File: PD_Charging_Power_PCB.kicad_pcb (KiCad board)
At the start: 2 copper layers, 30 x 28 mm, 35 parts, among them J1 105450-0101, Q1 CJQ4459, Q2 2N7002KDW, U1 STUSB4500

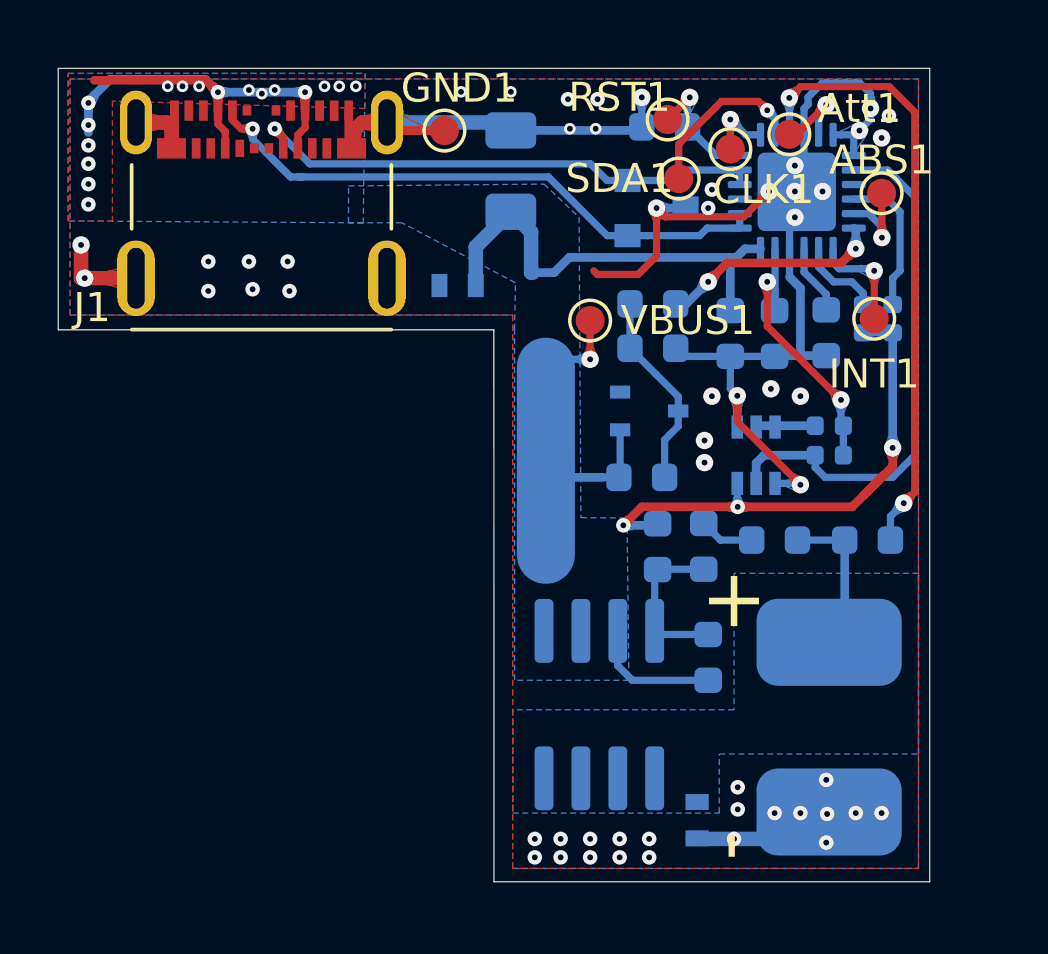
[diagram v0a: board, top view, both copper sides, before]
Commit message: Ruan: V0.3
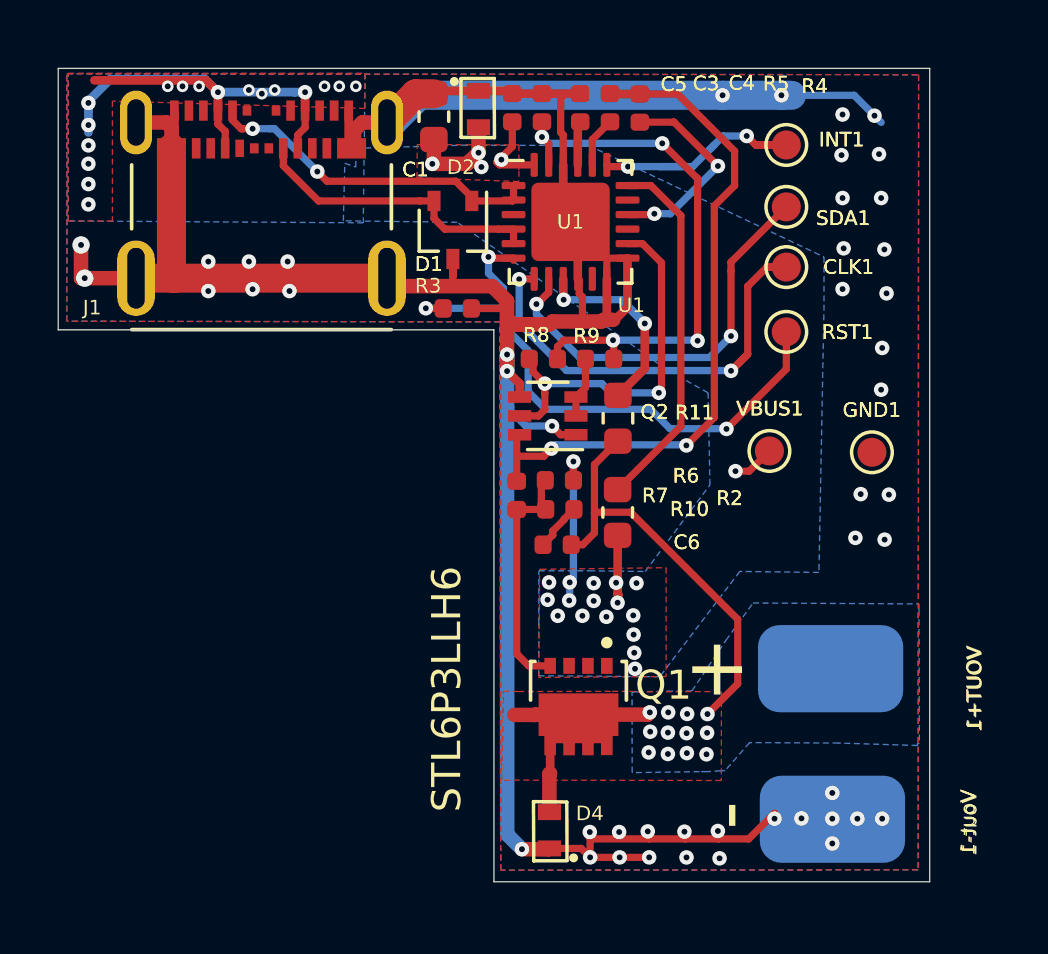
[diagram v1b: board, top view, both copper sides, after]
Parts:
- removed ABS1: ABS, TestPoint:TestPoint_Pad_D1.0mm
- removed Att1: ATT, TestPoint:TestPoint_Pad_D1.0mm
- removed C2: 1uF, Capacitor_SMD:C_0603_1608Metric
- removed D3: BAT54W, Package_TO_SOT_SMD:SOT-323_SC-70
- removed R1: 470R, Resistor_SMD:R_0603_1608Metric
- C1: footprint Capacitor_SMD:C_1206_3216Metric -> Capacitor_SMD:C_0603_1608Metric; moved to F.Cu
- C3, C4, C5, C6: footprint Capacitor_SMD:C_0603_1608Metric -> Capacitor_SMD:C_0402_1005Metric; moved to F.Cu
- D1: value ESD24VC2 -> ESDA25W; footprint Package_TO_SOT_SMD:SOT-23 -> Package_TO_SOT_SMD:SOT-323_SC-70; moved to F.Cu
- D2, D4, Q2, R11, R2, R4, R5, R8, R9, U1: moved to F.Cu
- Q1: value CJQ4459 -> STL6P3LLH6; footprint RuanProject:SOP-8_CJQ4459 -> RuanProject:PowerFLAT-3x3mm-8pin; moved to F.Cu
- R10, R3, R6, R7: footprint Resistor_SMD:R_0603_1608Metric -> Resistor_SMD:R_0402_1005Metric; moved to F.Cu
- moved GND1 18.4 mm to (63.2, 150.3)
- moved C4 11.5 mm to (53.1, 138.4), turned to 270 degrees
- moved R5 11.3 mm to (54.2, 138.4), turned to 270 degrees
- moved R4 11.3 mm to (55.2, 138.4), turned to 270 degrees
- moved C3 11.2 mm to (51.8, 138.4), turned to 270 degrees
- moved C5 10.8 mm to (50.8, 138.4), turned to 270 degrees
- moved R8 10.4 mm to (51.9, 147.1)
- moved R11 9.56 mm to (54.4, 149.1), turned to 90 degrees
- moved R3 9.49 mm to (48.9, 145.3), turned to 0 degrees
- moved RST1 8.37 mm to (60.2, 146.1)
- moved R9 8.23 mm to (53.8, 147.1)
- moved R6 7.96 mm to (52.4, 151.2), turned to 180 degrees
- moved U1 7.86 mm to (52.8, 142.3)
- moved VBUS1 7.63 mm to (59.6, 150.2)
- moved C6 7.49 mm to (52.3, 153.4)
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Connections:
- R2 pad 1: Net-(C2-Pad1) -> VBUS
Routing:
- net GND: track 64.4 -> 122.9 mm, vias 54 -> 47
- net VBUS: track 51.2 -> 33.0 mm, vias 18 -> 39
- net Net-(R3-Pad1): track 4.33 -> 21.0 mm, vias 1 -> 3
- net Net-(C6-Pad1): track 6.71 -> 23.0 mm, vias 0 -> 12
- net Net-(R11-Pad2): track 21.2 -> 6.71 mm
- net Net-(CLK1-Pad1): track 2.27 -> 16.2 mm, vias 1 -> 2
- net /CC1: track 21.5 -> 11.8 mm, vias 1 -> 2
- net +2V8: track 10.3 -> 19.1 mm, vias 2 -> 4
- net Net-(SDA1-Pad1): track 5.92 -> 14.3 mm, vias 1 -> 2
- net /CC2: track 18.2 -> 10.3 mm, vias 1 -> 0
- net Net-(C2-Pad1): track 6.85 -> 0.00 mm
- net Net-(Q2-Pad5): track 18.5 -> 12.8 mm, vias 0 -> 2
- net Net-(INT1-Pad1): track 3.66 -> 9.04 mm, vias 1 -> 2
- net Net-(R2-Pad2): track 7.76 -> 12.6 mm, vias 2 -> 0
- net Net-(Q2-Pad6): track 19.6 -> 23.6 mm, vias 3 -> 2
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- added copper zone on F.Cu, net Net-(C6-Pad1)

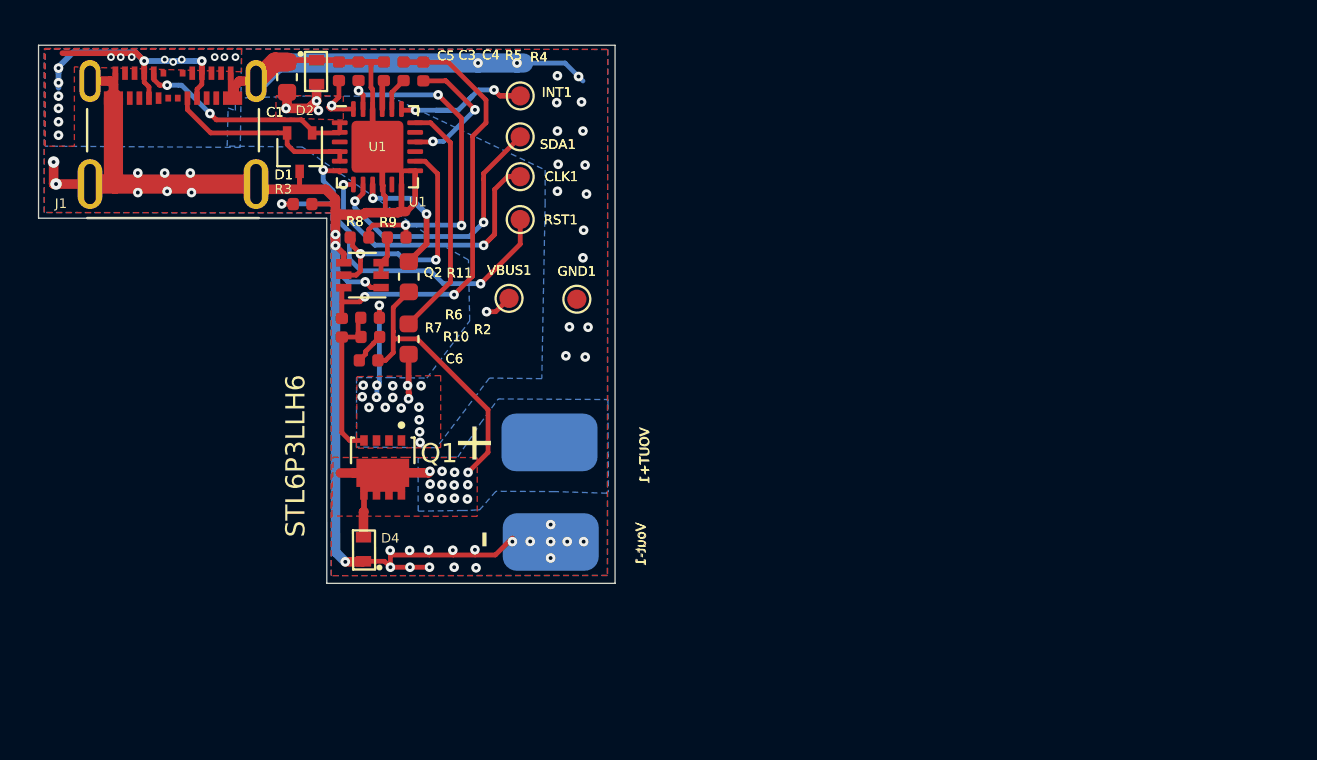
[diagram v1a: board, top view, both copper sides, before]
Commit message: Ruan: change to V0.5
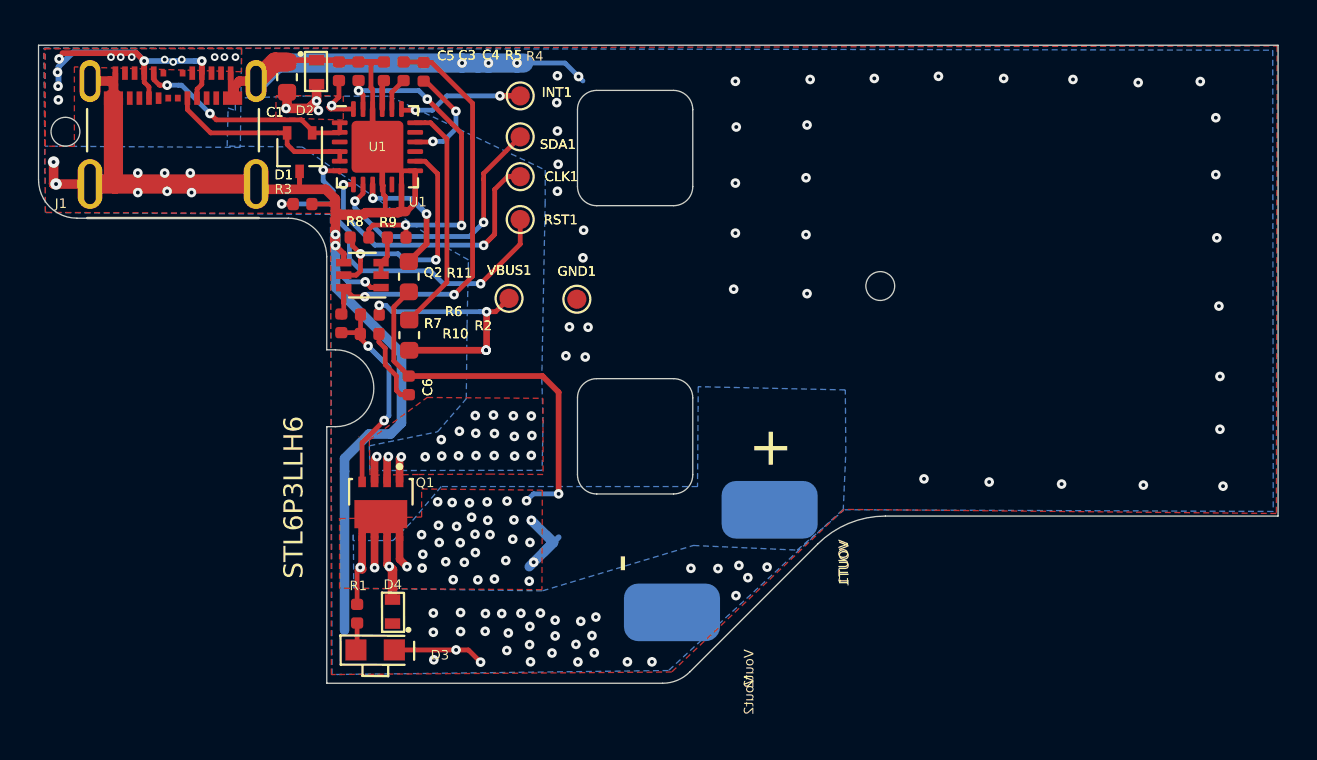
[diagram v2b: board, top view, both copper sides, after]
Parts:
- added D3: Power_LED, RuanProject:Led-LTST-S270KGKT, F.Cu at (53.7, 168.5)
- added R1: 2.2K, Resistor_SMD:R_0402_1005Metric, F.Cu at (51.7, 166.6)
- Q2: value 2N7002KDW -> 2N7002KDW (NC)
- R4: value 0R(NC) -> 0R
- R8: value 10K -> 10K(NC)
- R9: value 10K -> 10K (NC)
- moved VOUT1 12.0 mm to (73.1, 161.3)
- moved Vout2 7.29 mm to (68.0, 166.6)
- moved D4 3.58 mm to (53.6, 165.9)
- moved C6 2.46 mm to (54.4, 154.7), turned to 270 degrees
- moved Q1 2.16 mm to (53.0, 161.3)
- moved R7 0.23 mm to (50.9, 151.5)
- moved R2 0.21 mm to (54.4, 152.1)
- moved R6 0.17 mm to (52.4, 151.1)
- moved R10 0.16 mm to (52.4, 152.1)
- renumbered VOUT+1 to VOUT1, Vout-1 to Vout2
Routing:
- net Net-(C6-Pad1): track 23.0 -> 37.1 mm, vias 12 -> 35
- net VBUS: track 33.0 -> 41.8 mm, vias 39 -> 43
- net Net-(Q1-Pad4): track 8.34 -> 12.6 mm, vias 0 -> 2
- net Net-(C6-Pad2): track 1.66 -> 4.05 mm
- net Net-(INT1-Pad1): track 9.04 -> 7.39 mm
- net Net-(R4-Pad2): track 7.12 -> 5.64 mm
- net Net-(D3-Pad2): track 0.00 -> 1.43 mm
- net GND: track 122.9 -> 122.4 mm, vias 47 -> 87
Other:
- board size 30 x 28 mm -> 64.5 x 33.2 mm
